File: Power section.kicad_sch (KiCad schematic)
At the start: 17 parts, among them J2 USB3_A, U4 TLV76733, U5 USBLC6-2P6, U6 TPS7A0212

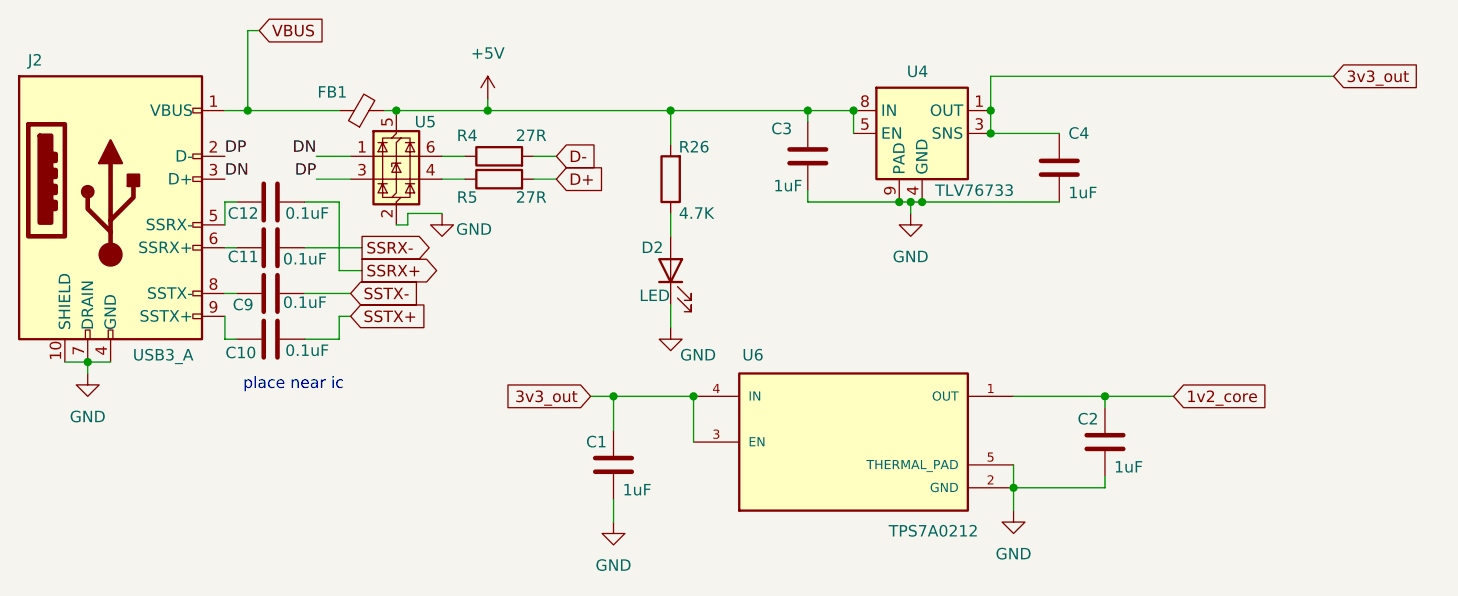
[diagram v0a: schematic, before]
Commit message: merged with main branch, no major change in pcb or schematics
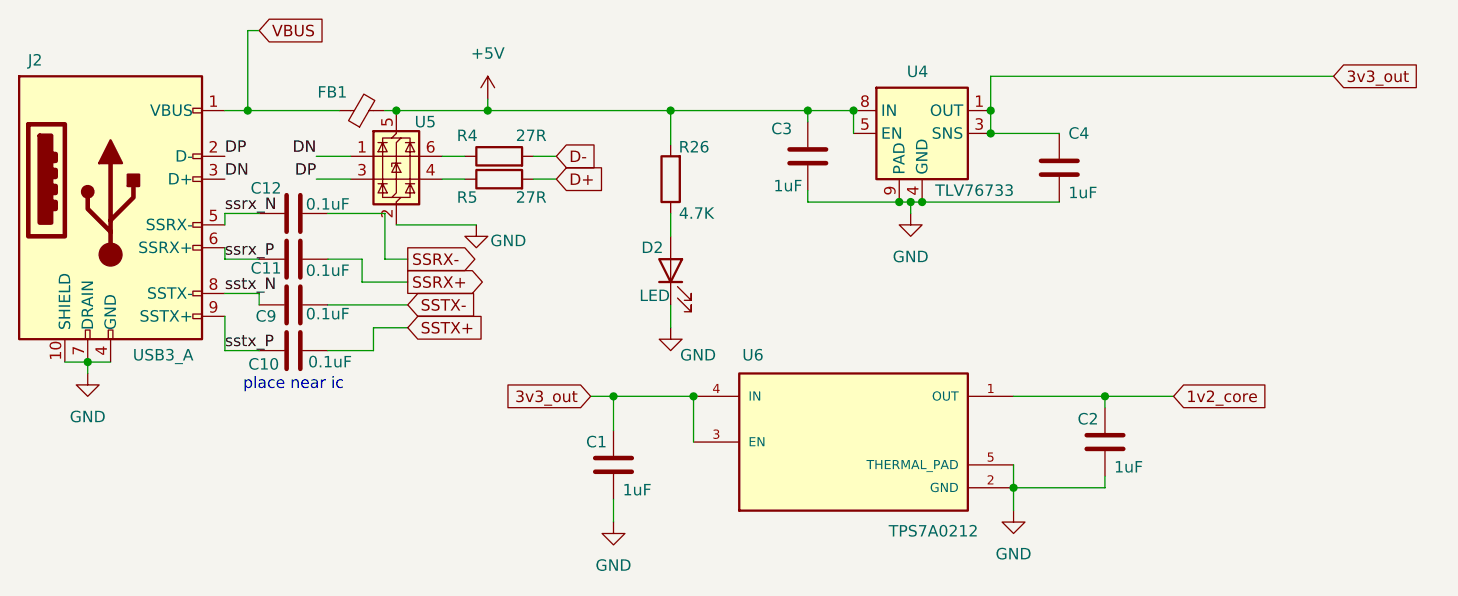
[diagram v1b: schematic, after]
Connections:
- net SSRX+: now also C11.2; no longer C12.2
- net SSRX-: now also C12.2; no longer C11.2
- net sstx_N: now reaches C9.1, J2.8 (SSTX-)
- net ssrx_N: now reaches C12.1, J2.5 (SSRX-)
- net ssrx_P: now reaches C11.1, J2.6 (SSRX+)
- net sstx_P: now reaches C10.1, J2.9 (SSTX+)
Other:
- moved on the sheet: C10, C11, C12, C9
